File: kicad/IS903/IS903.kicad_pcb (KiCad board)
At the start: 4 copper layers, 33 x 14 mm, 31 parts, among them J1 USB3_A, U1 IS903_QFN64_8*8, U2 EML3020, U3 EMP8733-1.2, U4 NAND_BGA152, U5 NAND_BGA152, Y1 30MHZ 2520

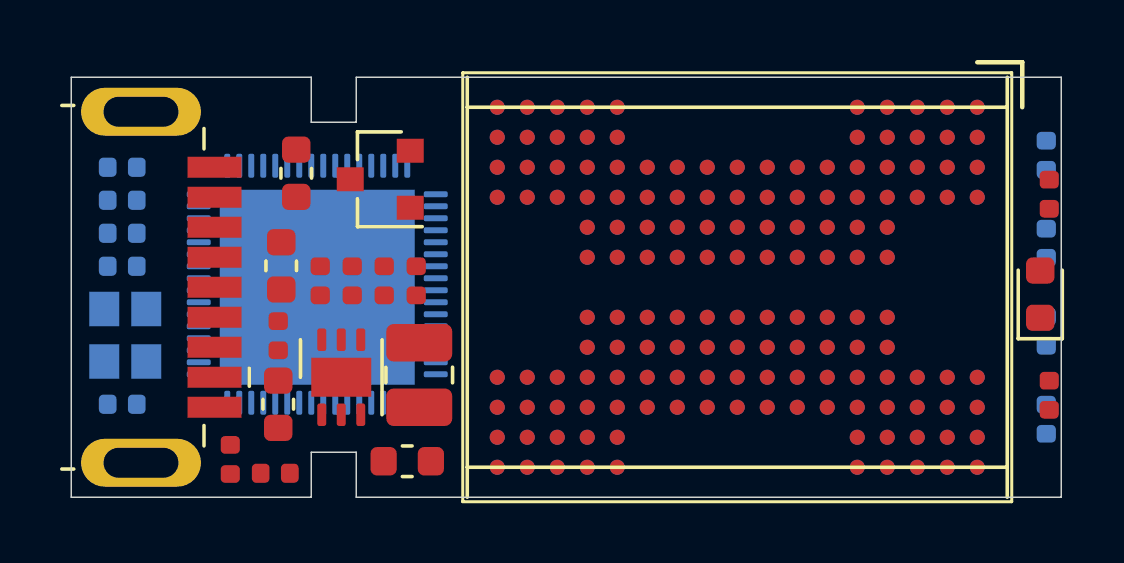
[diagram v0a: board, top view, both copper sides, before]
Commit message: 2020.7.23
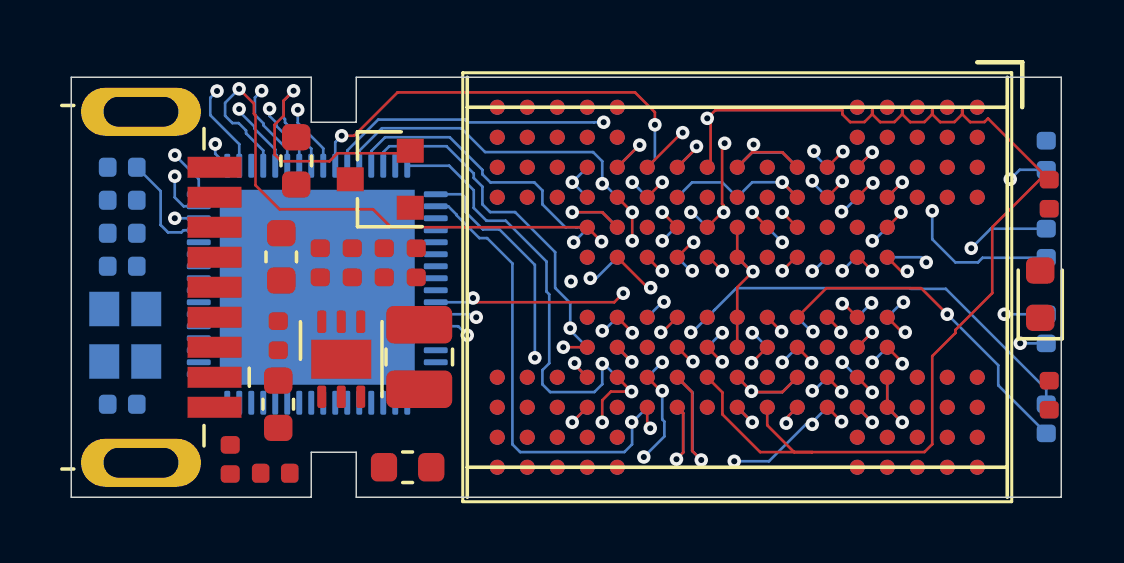
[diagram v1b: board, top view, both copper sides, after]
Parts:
- moved R8 3.02 mm to (132.5, 94.4)
- moved R7 2.92 mm to (132.5, 97.4)
- moved C11 0.60 mm to (111.5, 92.2)
- moved C8 0.60 mm to (108.3, 92.2)
- moved L1 0.60 mm to (111.6, 95.3)
- moved R1 0.60 mm to (109.4, 92.2)
- moved R2 0.60 mm to (110.4, 92.2)
- moved U2 0.60 mm to (109.0, 95.4)
- moved C7 0.41 mm to (107.5, 88.8)
- moved C9 0.30 mm to (107.0, 92.0)
- moved C5 0.20 mm to (111.2, 99.0)
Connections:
- U1 pad 30: Net-(U1-Pad30) -> (no net)
- U1 pad 31: Net-(U1-Pad31) -> (no net)
- U1 pad 32: Net-(U1-Pad32) -> (no net)
- U1 pad 5: Net-(U1-Pad5) -> (no net)
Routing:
- net /VSS1: track 0.00 -> 38.5 mm, vias 0 -> 1
- net /F0_IO3: track 0.00 -> 37.4 mm, vias 0 -> 3
- net /F0_IO0: track 0.00 -> 37.4 mm, vias 0 -> 4
- net /F0_IO1: track 0.00 -> 33.2 mm, vias 0 -> 4
- net /F0_IO5: track 0.00 -> 32.8 mm, vias 0 -> 4
- net /F0_IO2: track 0.00 -> 32.1 mm, vias 0 -> 4
- net /F0_IO4: track 0.00 -> 29.3 mm, vias 0 -> 3
- net +3V3: track 0.00 -> 27.7 mm, vias 0 -> 10
- net GND: track 0.00 -> 27.5 mm, vias 0 -> 13
- net Net-(R4-Pad1): track 0.00 -> 27.3 mm, vias 0 -> 2
- net /F0_IO6: track 0.00 -> 25.9 mm, vias 0 -> 3
- net /F0_IO7: track 0.00 -> 25.9 mm, vias 0 -> 3
- net /F1_IO5: track 0.00 -> 24.9 mm, vias 0 -> 2
- net /F1_IO4: track 0.00 -> 24.4 mm, vias 0 -> 2
- net /F1_IO7: track 0.00 -> 23.6 mm, vias 0 -> 2
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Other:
- rule via_min_drill: 0.00508 -> 0.2
- rule via_min_size: 0.01143 -> 0.45
